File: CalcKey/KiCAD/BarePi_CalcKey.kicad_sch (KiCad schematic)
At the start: 51 parts, among them J1 IN, J2 OUT, J3 WCH-LINK, U1 CH32V002F4P6

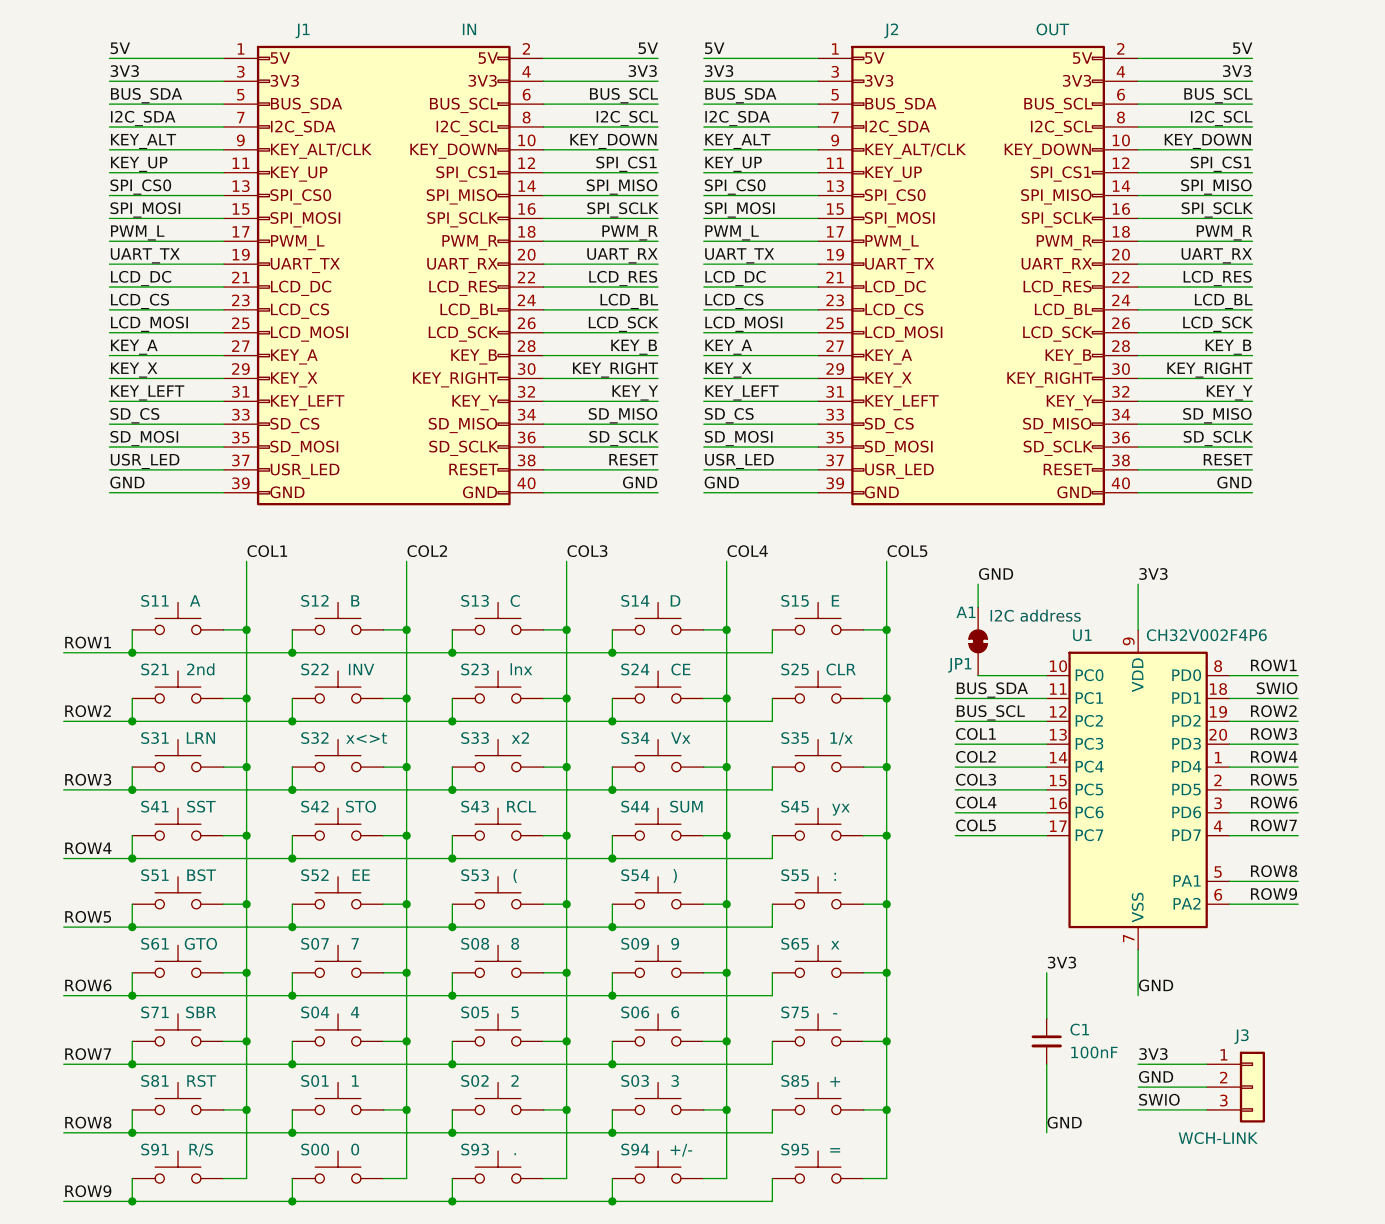
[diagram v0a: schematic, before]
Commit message: init
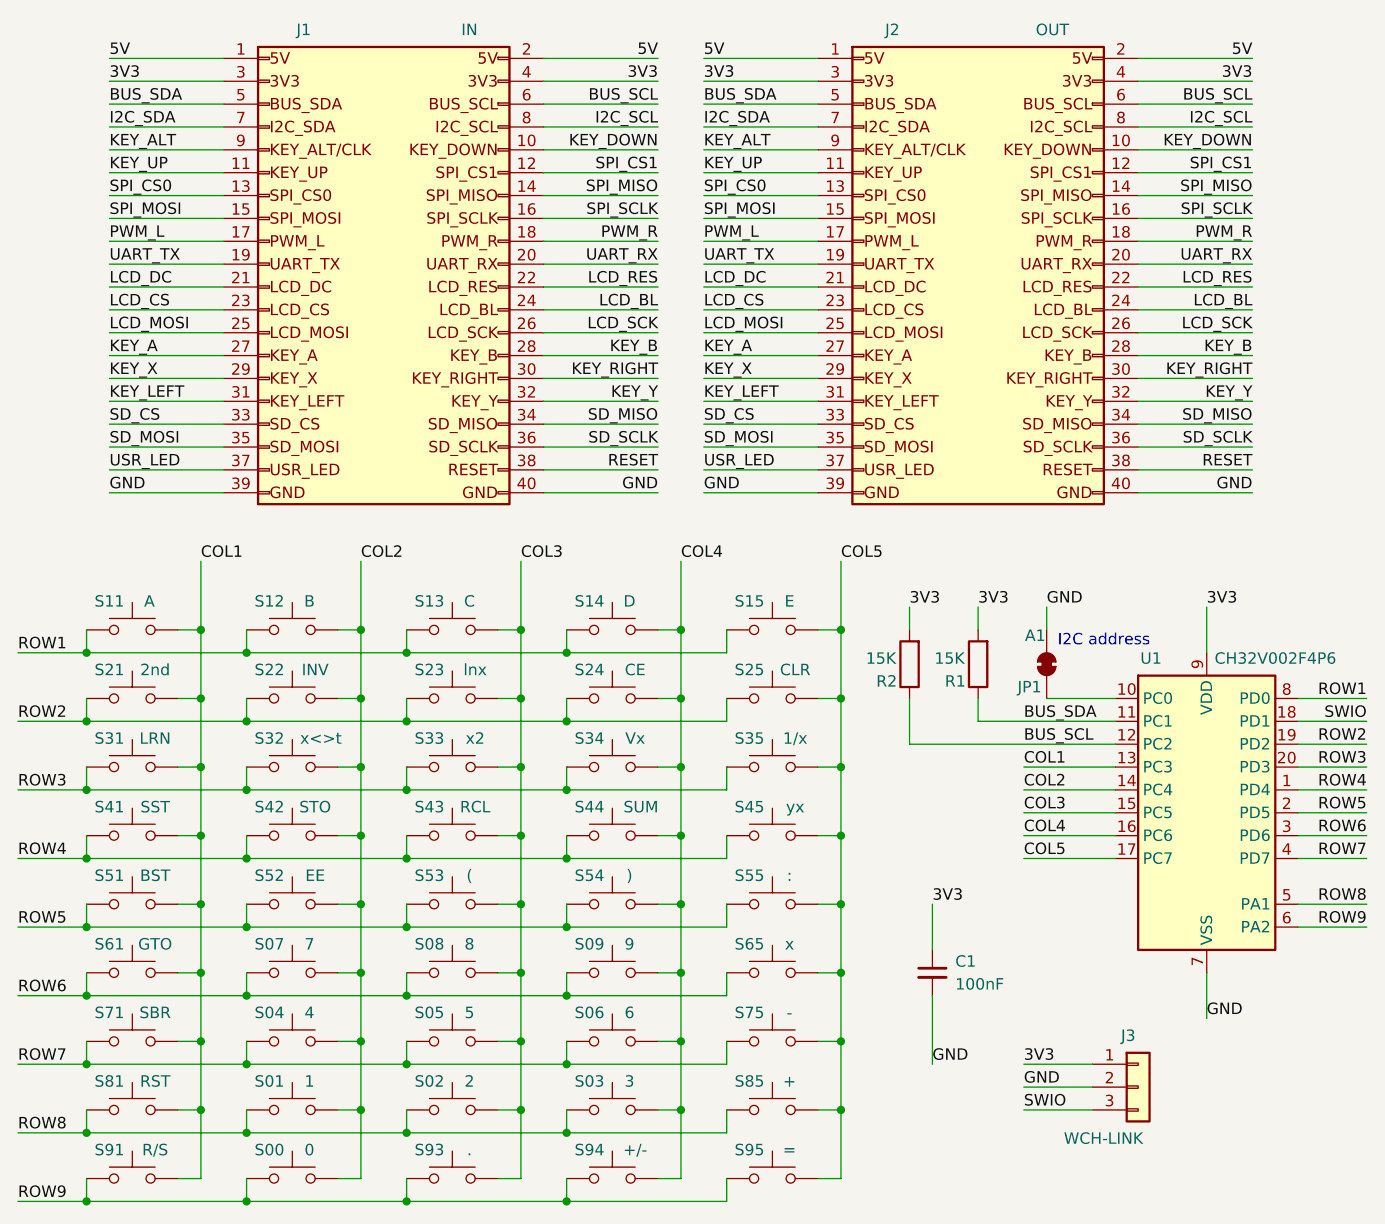
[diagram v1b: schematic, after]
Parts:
- added R1, R2: 15K, Resistor_SMD:R_1206_3216Metric_Pad1.30x1.75mm_HandSolder, symbol Device:R
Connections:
- net 3V3: now also R1.2, R2.2
- net BUS_SCL: now also R2.1
- net BUS_SDA: now also R1.1
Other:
- moved on the sheet: C1, J3, JP1, S00, S01, S02, S03, S04, S05, S06, S07, S08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
